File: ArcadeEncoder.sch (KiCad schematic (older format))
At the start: 3 parts, among them J1 DB15_Male, J2 DB9_Male, U1 ProMicro

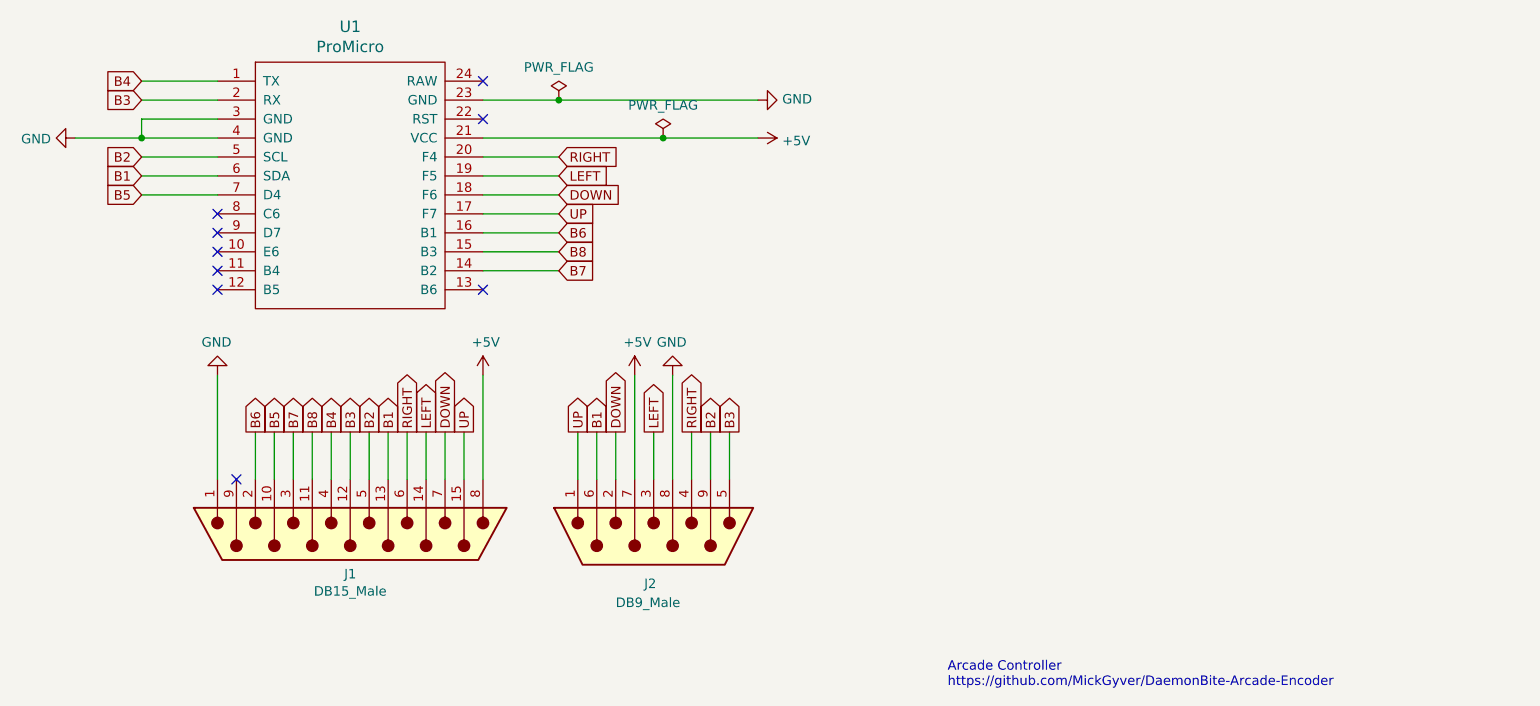
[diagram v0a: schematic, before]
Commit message: Changes for sega
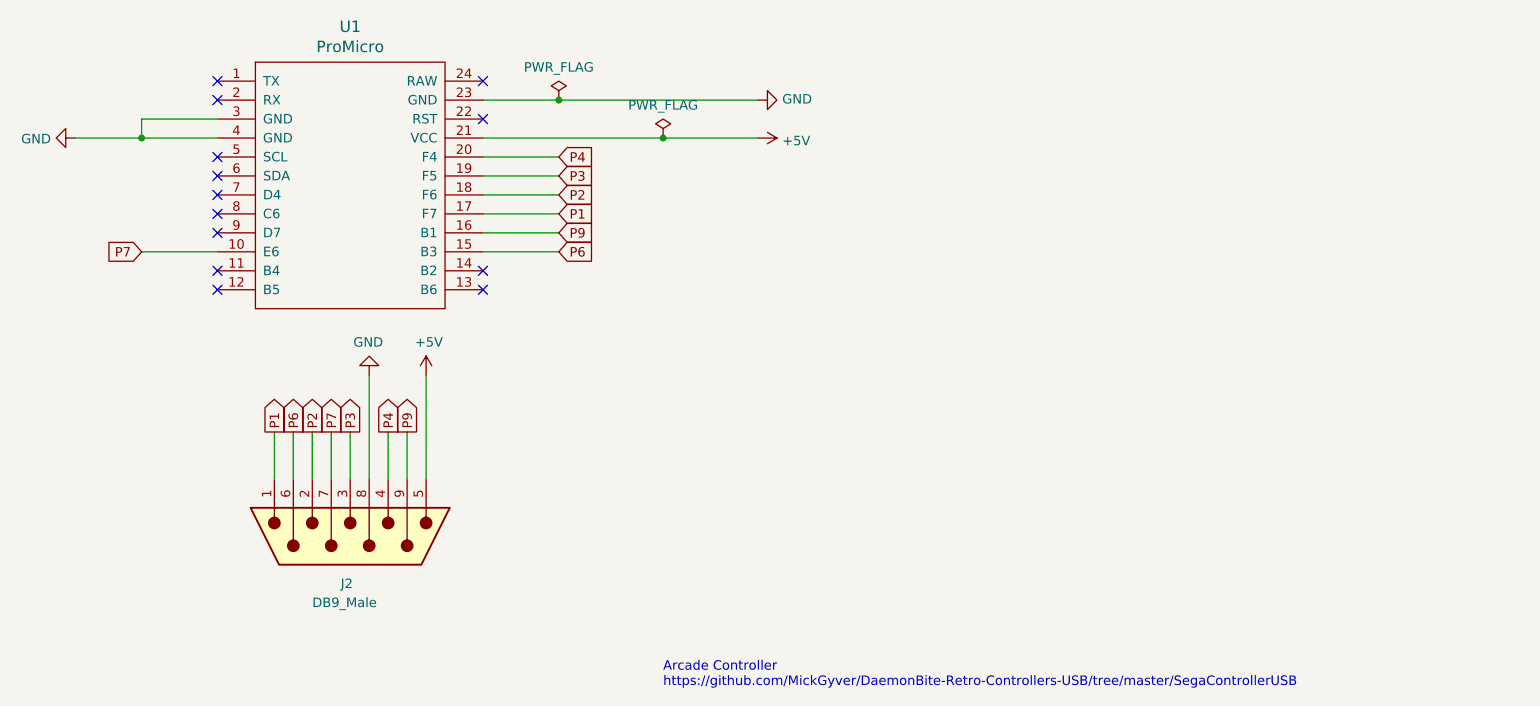
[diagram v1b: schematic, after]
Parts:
- removed J1: DB15_Male, halibs:D-Sub_Connector_15P-Male, symbol Connector:DB15_Male
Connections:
- net +5V: now also J2.5; no longer J2.7
- net P7: now reaches U1.10 (E6)
- net P7: now also J2.7
- net B1: no longer names the net of U1.6 (SDA)
- net B1: no longer J2.6
- net B2: no longer names the net of U1.5 (SCL)
- net B2: no longer J2.9
- net B3: no longer names the net of U1.2 (RX)
- net B3: no longer J2.5
- net B4: no longer names the net of U1.1 (TX)
- net B5: no longer names the net of U1.7 (D4)
- net B6 renamed P9
- net P9: now also J2.9
- net B7: no longer names the net of U1.14 (B2)
- net B8 renamed P6
- net P6: now also J2.6
- net DOWN renamed P2
- net LEFT renamed P3
- net RIGHT renamed P4
- net UP renamed P1
- no-connect marks 9 -> 13
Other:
- note added: "Arcade Controller\nhttps://github.com/MickGyver/DaemonBite-Retro-Controllers-USB/tree/master/SegaControllerUSB"
- note removed: "Arcade Controller\nhttps://github.com/MickGyver/DaemonBite-Arcade-Encoder"
- moved on the sheet: J2
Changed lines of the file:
@@
 encoding utf-8
 Sheet 1 1
-Title "Arcade-Encoder"
-Date "2020-11-05"
-Rev "0.2"
+Title "Arcade-Encoder (Sega)"
+Date "2020-11-19"
+Rev "0.1"
 Comp "haus-automatisierung.com"
 Comment1 ""
@@
 	1    0    0    -1
 $EndComp
-$Comp
-L Connector:DB15_Male J1
-U 1 1 5FA46F7A
-P 5600 5650
-F 0 "J1" V 5799 5650 50  0000 C CNN
-F 1 "DB15_Male" V 5890 5650 50  0000 C CNN
-F 2 "halibs:D-Sub_Connector_15P-Male" H 5600 5650 50  0001 C CNN
-F 3 " ~" H 5600 5650 50  0001 C CNN
-	1    5600 5650
-	0    1    1    0
-$EndComp
-$Comp
-L power:+5V #PWR03
-U 1 1 5FA4B57F
-P 6300 4800
-F 0 "#PWR03" H 6300 4650 50  0001 C CNN
-F 1 "+5V" H 6315 4973 50  0000 C CNN
-F 2 "" H 6300 4800 50  0001 C CNN
-F 3 "" H 6300 4800 50  0001 C CNN
-	1    6300 4800
-	1    0    0    -1
-$EndComp
-Wire Wire Line
-	6300 4800 6300 5350
 $Comp
 L power:+5V #PWR05
@@
 	0    1    1    0
 $EndComp
-$Comp
-L power:GND #PWR02
-U 1 1 5FA4CDB2
-P 4900 4800
-F 0 "#PWR02" H 4900 4550 50  0001 C CNN
-F 1 "GND" H 4905 4627 50  0000 C CNN
-F 2 "" H 4900 4800 50  0001 C CNN
-F 3 "" H 4900 4800 50  0001 C CNN
-	1    4900 4800
-	-1   0    0    1
-$EndComp
-Wire Wire Line
-	4900 5350 4900 4800
-Text GLabel 4500 3250 0    50   Input ~ 0
-B4
-Wire Wire Line
-	4500 3250 4900 3250
-Text GLabel 5500 5100 1    50   Output ~ 0
-B4
-Wire Wire Line
-	5500 5100 5500 5350
-Text GLabel 4500 3350 0    50   Input ~ 0
-B3
-Wire Wire Line
-	4500 3350 4900 3350
-Text GLabel 5600 5100 1    50   Output ~ 0
-B3
-Wire Wire Line
-	5600 5100 5600 5350
 NoConn ~ 6300 3250
 NoConn ~ 6300 3450
-NoConn ~ 4900 4150
 NoConn ~ 4900 3950
 $Comp
@@
 Wire Wire Line
 	6700 3350 7750 3350
-Text GLabel 4500 3650 0    50   Input ~ 0
-B2
-Wire Wire Line
-	4500 3650 4900 3650
-Text GLabel 4500 3750 0    50   Input ~ 0
-B1
-Wire Wire Line
-	4500 3750 4900 3750
-Text GLabel 4500 3850 0    50   Input ~ 0
-B5
-Wire Wire Line
-	4500 3850 4900 3850
 Text GLabel 6700 3650 2    50   Input ~ 0
-RIGHT
+P4
 Wire Wire Line
 	6700 3650 6300 3650
-Text GLabel 6700 3750 2    50   Input ~ 0
-LEFT
-Wire Wire Line
-	6700 3750 6300 3750
-Text GLabel 6700 3850 2    50   Input ~ 0
-DOWN
-Wire Wire Line
-	6700 3850 6300 3850
-Text GLabel 6700 3950 2    50   Input ~ 0
-UP
-Wire Wire Line
-	6700 3950 6300 3950
-Text GLabel 6700 4050 2    50   Input ~ 0
-B6
-Wire Wire Line
-	6700 4050 6300 4050
-Text GLabel 6700 4150 2    50   Input ~ 0
-B8
-Wire Wire Line
-	6700 4150 6300 4150
-Text GLabel 6700 4250 2    50   Input ~ 0
-B7
-Wire Wire Line
-	6700 4250 6300 4250
-Text GLabel 5100 5100 1    50   Output ~ 0
-B6
-Wire Wire Line
-	5100 5100 5100 5350
-Text GLabel 5700 5100 1    50   Output ~ 0
-B2
-Wire Wire Line
-	5700 5100 5700 5350
-Text GLabel 5900 5100 1    50   Output ~ 0
-RIGHT
-Wire Wire Line
-	5900 5100 5900 5350
-Text GLabel 6100 5100 1    50   Output ~ 0
-DOWN
-Wire Wire Line
-	6100 5100 6100 5350
-NoConn ~ 5000 5350
-Text GLabel 5200 5100 1    50   Output ~ 0
-B5
-Wire Wire Line
-	5200 5100 5200 5350
-Text GLabel 5800 5100 1    50   Output ~ 0
-B1
-Wire Wire Line
-	5800 5100 5800 5350
-Text GLabel 6000 5100 1    50   Output ~ 0
-LEFT
-Wire Wire Line
-	6000 5100 6000 5350
-Text GLabel 6200 5100 1    50   Output ~ 0
-UP
-Wire Wire Line
-	6200 5100 6200 5350
-Text GLabel 5300 5100 1    50   Output ~ 0
-B7
-Wire Wire Line
-	5300 5100 5300 5350
-Text GLabel 5400 5100 1    50   Output ~ 0
-B8
-Wire Wire Line
-	5400 5100 5400 5350
 $Comp
 L power:GND #PWR0102
@@
 L Connector:DB9_Male J2
 U 1 1 5FA50C79
-P 7200 5650
-F 0 "J2" V 7450 5600 50  0000 L CNN
-F 1 "DB9_Male" V 7550 5450 50  0000 L CNN
-F 2 "halibs:D-Sub_Connector_9P-Male" H 7200 5650 50  0001 C CNN
-F 3 " ~" H 7200 5650 50  0001 C CNN
-	1    7200 5650
+P 5600 5650
+F 0 "J2" V 5850 5600 50  0000 L CNN
+F 1 "DB9_Male" V 5950 5450 50  0000 L CNN
+F 2 "halibs:D-Sub_Connector_9P-Male" H 5600 5650 50  0001 C CNN
+F 3 " ~" H 5600 5650 50  0001 C CNN
+	1    5600 5650
 	0    1    1    0
 $EndComp
-Text GLabel 6800 5100 1    50   Output ~ 0
-UP
-Wire Wire Line
-	6800 5100 6800 5350
-Text GLabel 7000 5100 1    50   Output ~ 0
-DOWN
-Wire Wire Line
-	7000 5100 7000 5350
-Text GLabel 7200 5100 1    50   Output ~ 0
-LEFT
-Wire Wire Line
-	7200 5100 7200 5350
-Text GLabel 7600 5100 1    50   Output ~ 0
-B3
-Wire Wire Line
-	7600 5100 7600 5350
+Text GLabel 5200 5100 1    50   Output ~ 0
+P1
+Wire Wire Line
+	5200 5100 5200 5350
+Wire Wire Line
+	5400 5100 5400 5350
+Wire Wire Line
+	5600 5100 5600 5350
 $Comp
 L power:GND #PWR04
 U 1 1 5FA569FD
-P 7300 4800
-F 0 "#PWR04" H 7300 4550 50  0001 C CNN
-F 1 "GND" H 7305 4627 50  0000 C CNN
-F 2 "" H 7300 4800 50  0001 C CNN
-F 3 "" H 7300 4800 50  0001 C CNN
-	1    7300 4800
+P 5700 4800
+F 0 "#PWR04" H 5700 4550 50  0001 C CNN
+F 1 "GND" H 5705 4627 50  0000 C CNN
+F 2 "" H 5700 4800 50  0001 C CNN
+F 3 "" H 5700 4800 50  0001 C CNN
+	1    5700 4800
 	-1   0    0    1
 $EndComp
 Wire Wire Line
-	7300 4800 7300 5350
+	5700 4800 5700 5350
 $Comp
 L power:+5V #PWR01
 U 1 1 5FA578A0
-P 7100 4800
-F 0 "#PWR01" H 7100 4650 50  0001 C CNN
-F 1 "+5V" H 7115 4973 50  0000 C CNN
-F 2 "" H 7100 4800 50  0001 C CNN
-F 3 "" H 7100 4800 50  0001 C CNN
-	1    7100 4800
-	1    0    0    -1
-$EndComp
-Wire Wire Line
-	7100 4800 7100 5350
-Text GLabel 7500 5100 1    50   Output ~ 0
-B2
-Wire Wire Line
-	7500 5100 7500 5350
-Text GLabel 6900 5100 1    50   Output ~ 0
-B1
-Wire Wire Line
-	6900 5100 6900 5350
-Text GLabel 7400 5100 1    50   Output ~ 0
-RIGHT
-Wire Wire Line
-	7400 5100 7400 5350
-Text Notes 8750 6450 0    50   ~ 0
-Arcade Controller\nhttps://github.com/MickGyver/DaemonBite-Arcade-Encoder
+P 6000 4800
+F 0 "#PWR01" H 6000 4650 50  0001 C CNN
+F 1 "+5V" H 6015 4973 50  0000 C CNN
+F 2 "" H 6000 4800 50  0001 C CNN
+F 3 "" H 6000 4800 50  0001 C CNN
+	1    6000 4800
+	1    0    0    -1
+$EndComp
+Wire Wire Line
+	5300 5100 5300 5350
+Wire Wire Line
+	5800 5100 5800 5350
+Text Notes 7250 6450 0    50   ~ 0
+Arcade Controller\nhttps://github.com/MickGyver/DaemonBite-Retro-Controllers-USB/tree/master/SegaControllerUSB
+NoConn ~ 6300 4250
+NoConn ~ 4900 3850
+NoConn ~ 4900 3750
+NoConn ~ 4900 3650
+NoConn ~ 4900 3350
+NoConn ~ 4900 3250
+Wire Wire Line
+	6000 4800 6000 5350
+Text GLabel 6700 3750 2    50   Input ~ 0
+P3
+Wire Wire Line
+	6700 3750 6300 3750
+Text GLabel 6700 3850 2    50   Input ~ 0
+P2
+Text GLabel 6700 3950 2    50   Input ~ 0
+P1
+Text GLabel 6700 4050 2    50   Input ~ 0
+P9
+Text GLabel 6700 4150 2    50   Input ~ 0
+P6
+Wire Wire Line
+	6300 3850 6700 3850
+Wire Wire Line
+	6300 3950 6700 3950
+Wire Wire Line
+	6700 4050 6300 4050
+Wire Wire Line
+	6300 4150 6700 4150
+Text GLabel 4500 4150 0    50   Input ~ 0
+P7
+Wire Wire Line
+	4500 4150 4900 4150
+Text GLabel 5300 5100 1    50   Output ~ 0
+P6
+Text GLabel 5400 5100 1    50   Output ~ 0
+P2
+Text GLabel 5500 5100 1    50   Output ~ 0
+P7
+Wire Wire Line
+	5500 5100 5500 5350
+Text GLabel 5600 5100 1    50   Output ~ 0
+P3
+Text GLabel 5800 5100 1    50   Output ~ 0
+P4
+Text GLabel 5900 5100 1    50   Output ~ 0
+P9
+Wire Wire Line
+	5900 5100 5900 5350
 $EndSCHEMATC
